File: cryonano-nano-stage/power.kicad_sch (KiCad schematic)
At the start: 36 parts, among them Q1 PMV100EPAR, U4 AP7363-33D-13

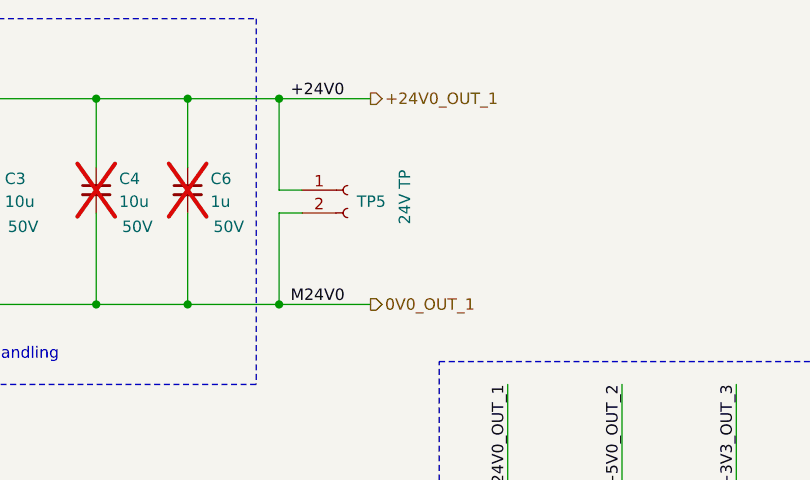
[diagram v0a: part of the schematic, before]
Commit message: release candidate
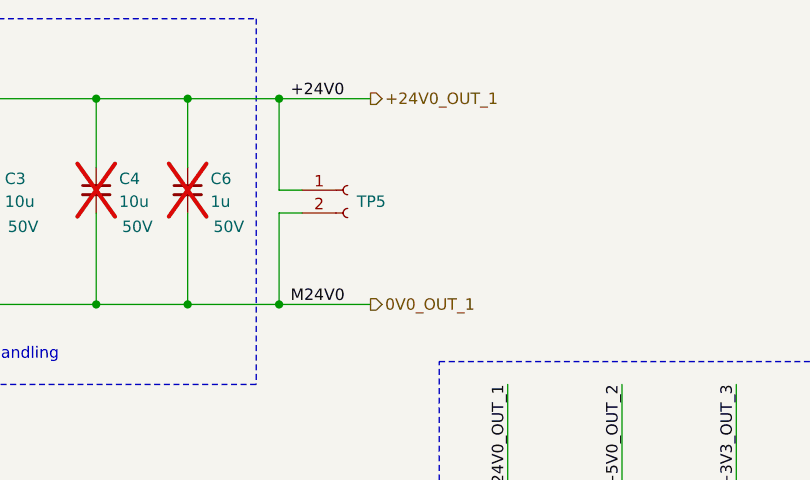
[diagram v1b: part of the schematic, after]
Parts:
- R1, R92, R93, R94: Order No. 0603/120mW -> 0603, 120mW
- R30: Order No. 0805/225mW -> 0805, 225mW
- TP1, TP4: Source N.A -> (none)
- TP5: Comment 24V TP -> (none)
